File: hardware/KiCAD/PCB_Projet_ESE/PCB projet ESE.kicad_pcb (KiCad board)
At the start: 4 copper layers, 53 x 46 mm, 82 parts, among them J1 Conn_01x06, J10 Conn_01x06, J11 Conn_01x06, J12 Conn_01x06, J13 Conn_01x06, J14 Conn_01x06, J15 Conn_01x06, J16 Conn_01x04, J2 Conn_01x04, J3 Conn_01x06, J4 Conn_01x03, J7 Conn_01x04, J8 Conn_01x02, J9 Conn_ST_STDC14, SW1 SW_SPST, SW2 472121010111, U1 ZXBM5210-SP, U2 ZXBM5210-SP, U3 STM32G474RETx, U4 ADXL343

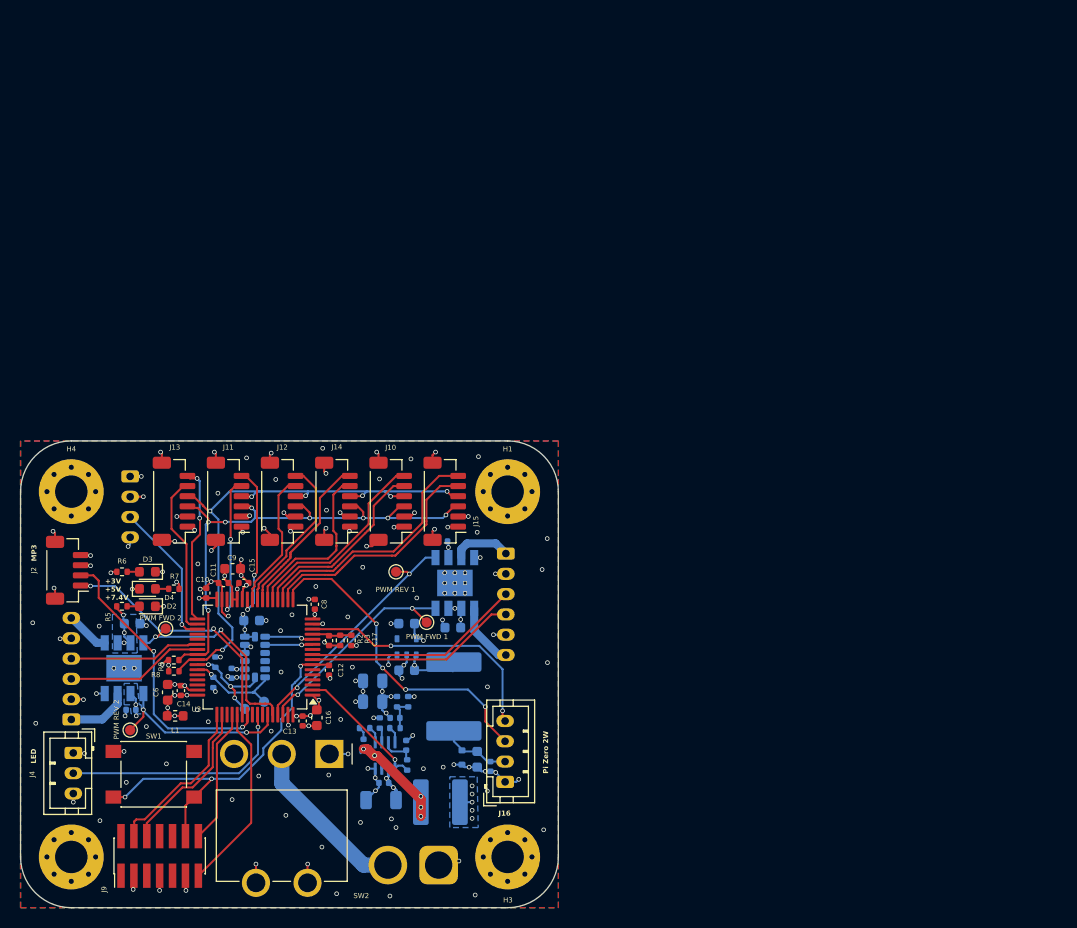
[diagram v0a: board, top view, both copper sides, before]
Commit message: v1.5 PCB finished
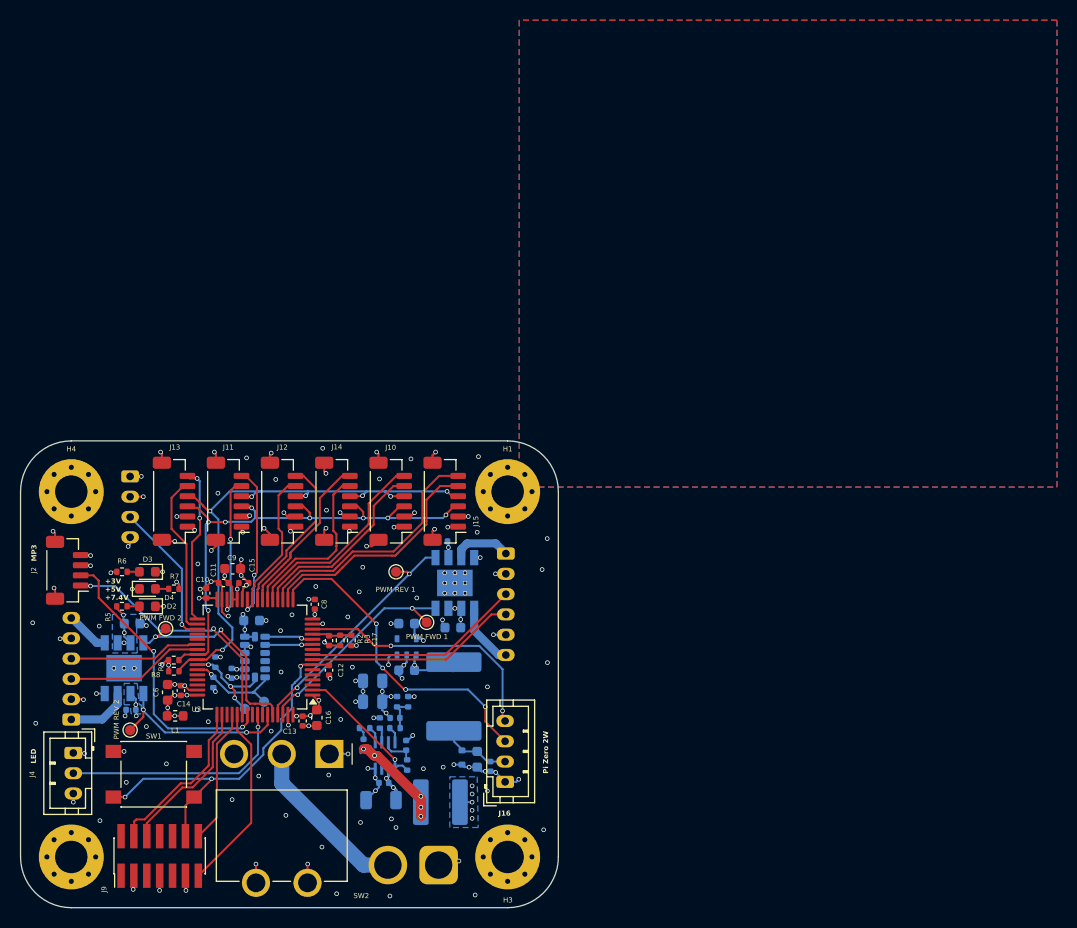
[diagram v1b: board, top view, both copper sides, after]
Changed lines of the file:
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@@
 		(polygon
 			(pts
-				(xy 132 54) (xy 79 54) (xy 79 100) (xy 132 100)
+				(xy 181.14 12.55) (xy 128.14 12.55) (xy 128.14 58.55) (xy 181.14 58.55)
 			)
 		)
@@
 		(polygon
 			(pts
-				(xy 132 54) (xy 79 54) (xy 79 100) (xy 132 100)
+				(xy 193.73 54.389293) (xy 140.73 54.389293) (xy 140.73 100.389293) (xy 193.73 100.389293)
 			)
 		)

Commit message: Finish README
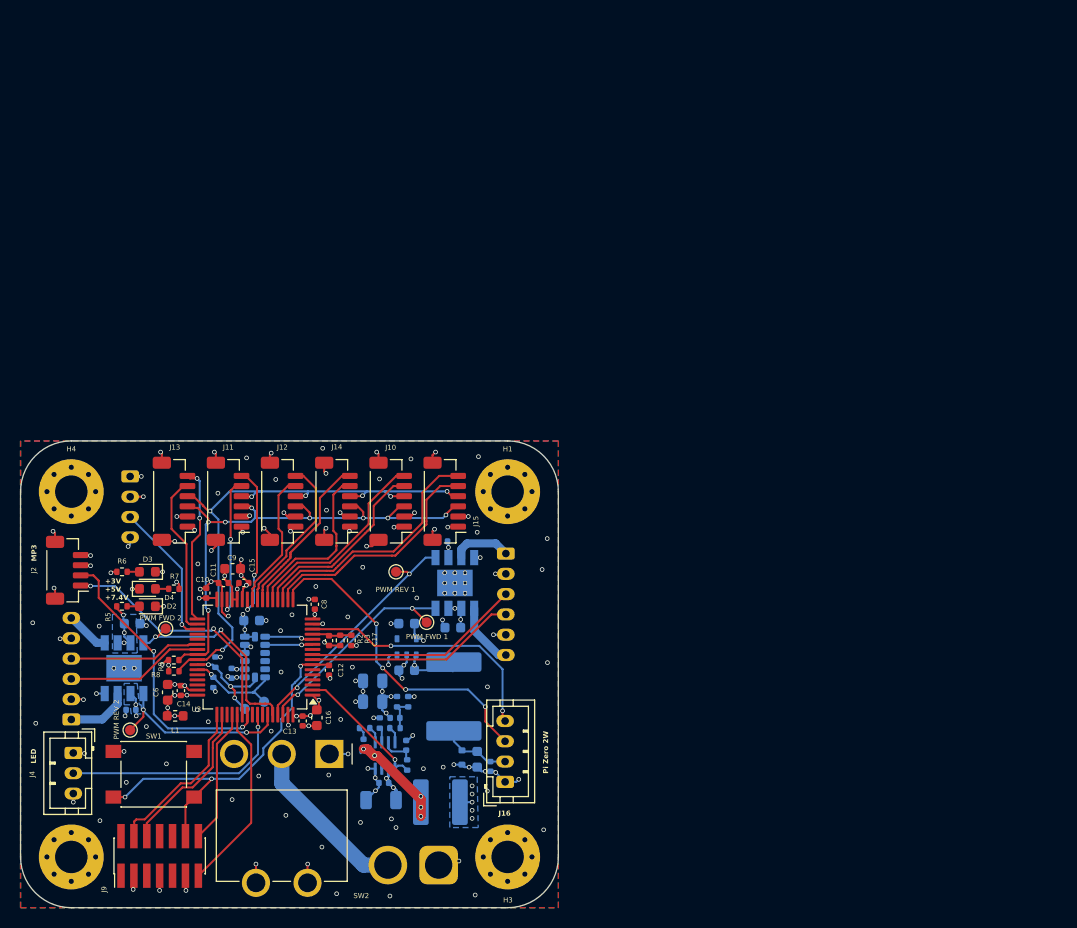
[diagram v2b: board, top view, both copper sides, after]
